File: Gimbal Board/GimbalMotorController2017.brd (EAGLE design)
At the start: 83.4 x 72.1 mm, 125 parts, among them J1 SL03THROUGH_HOLE, J3 APP_2POS_CONFIG5V_HORIZ, Q7 MOSFET-PCHANNEL, Q8 MOSFET-PCHANNEL, Q9 MOSFET-NCHANNELAO3404A, U1 NUP4201MR6, U2 MAX3232D, U3 CSD18533Q5A, U4 CSD18533Q5A, U5 CSD18533Q5A, U6 CSD18533Q5A, U7 CSD18533Q5A, U8 CSD18533Q5A

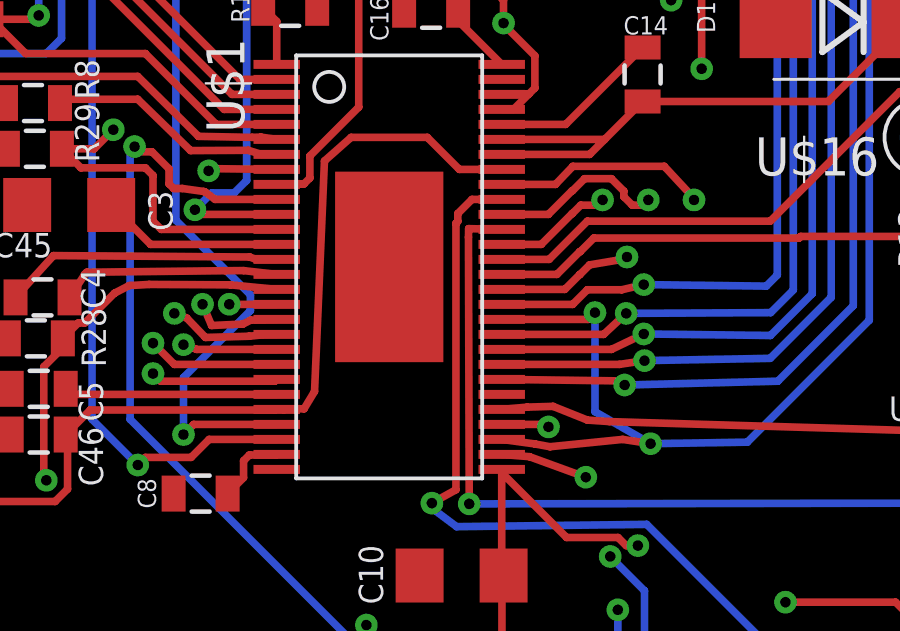
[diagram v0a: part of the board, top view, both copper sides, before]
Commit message: Board Updated for Board Review
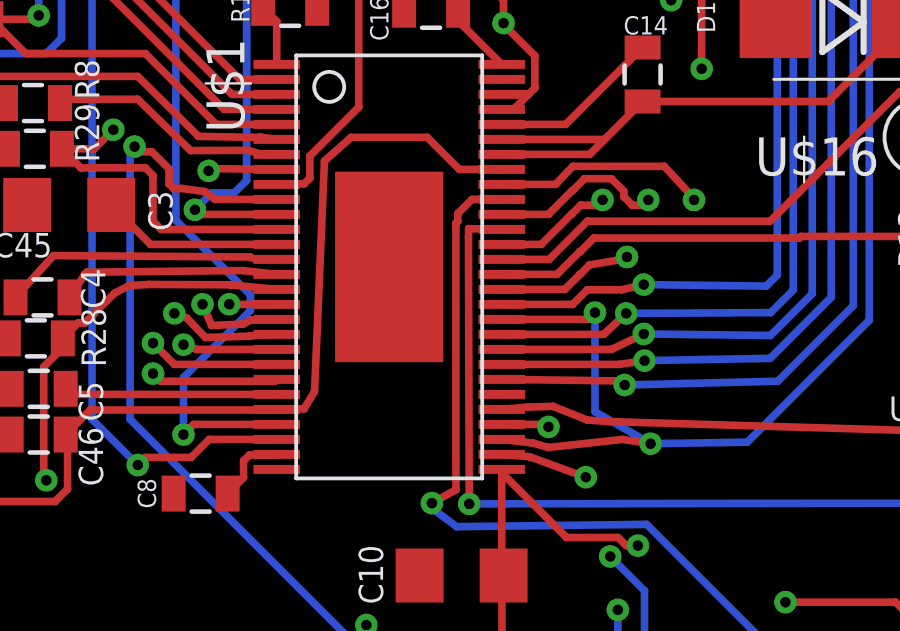
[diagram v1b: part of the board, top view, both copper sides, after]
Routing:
- net SDI: track 49.7 -> 48.9 mm
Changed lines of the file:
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@@
 <layers>
 <layer number="1" name="Top" color="4" fill="1" visible="yes" active="yes"/>
-<layer number="2" name="UpperMid" color="6" fill="1" visible="no" active="yes"/>
+<layer number="2" name="UpperMid" color="6" fill="1" visible="yes" active="yes"/>
 <layer number="3" name="Route3" color="4" fill="3" visible="no" active="no"/>
 <layer number="4" name="Route4" color="1" fill="4" visible="no" active="no"/>
@@
 <layer number="13" name="Route13" color="4" fill="5" visible="no" active="no"/>
 <layer number="14" name="Route14" color="1" fill="6" visible="no" active="no"/>
-<layer number="15" name="LowerMid" color="10" fill="1" visible="no" active="yes"/>
+<layer number="15" name="LowerMid" color="10" fill="1" visible="yes" active="yes"/>
 <layer number="16" name="Bottom" color="1" fill="1" visible="yes" active="yes"/>
 <layer number="17" name="Pads" color="2" fill="1" visible="yes" active="yes"/>
@@
 <wire x1="50.8" y1="3.81" x2="50.8" y2="4.80539375" width="0.254" layer="2"/>
 <wire x1="50.8" y1="4.80539375" x2="49.7078" y2="5.89759375" width="0.254" layer="2"/>
-<wire x1="49.7078" y1="5.89759375" x2="49.7078" y2="13.04436875" width="0.254" layer="2"/>
-<wire x1="49.7078" y1="13.04436875" x2="42.2176" y2="20.53456875" width="0.254" layer="2"/>
+<wire x1="49.7078" y1="5.89759375" x2="49.4538" y2="13.04436875" width="0.254" layer="2"/>
+<wire x1="49.4538" y1="13.04436875" x2="42.2176" y2="20.53456875" width="0.254" layer="2"/>
 <wire x1="42.2176" y1="27.8864" x2="42.164" y2="27.94" width="0.254" layer="2"/>
 <wire x1="42.2176" y1="20.53456875" x2="42.2176" y2="27.8864" width="0.254" layer="2"/>
@@
 <wire x1="47.32414375" y1="28.1698" x2="47.30434375" y2="28.15" width="0.254" layer="1"/>
 <wire x1="48.1552" y1="29.09754375" x2="48.1552" y2="28.363225" width="0.254" layer="1"/>
-<wire x1="47.961775" y1="28.1698" x2="47.0698" y2="28.1698" width="0.254" layer="1"/>
+<wire x1="47.32414375" y1="28.1698" x2="47.0698" y2="28.1698" width="0.254" layer="1"/>
 <wire x1="47.0698" y1="28.1698" x2="47.05" y2="28.15" width="0.254" layer="1"/>
 </signal>
@@
 <wire x1="73.8615" y1="45.43425" x2="73.8615" y2="47.01375" width="0.254" layer="1"/>
 <wire x1="73.50425" y1="47.371" x2="73.8615" y2="47.01375" width="0.254" layer="1"/>
-<wire x1="54.55" y1="19.65" x2="55.661" y2="19.4976" width="0.254" layer="1"/>
-<wire x1="55.661" y1="19.4976" x2="56.1594" y2="19.4056" width="0.254" layer="1"/>
-<wire x1="56.1594" y1="19.4056" x2="58.582" y2="19.65" width="0.254" layer="1"/>
+<wire x1="54.55" y1="19.65" x2="55.6102" y2="19.523" width="0.254" layer="1"/>
+<wire x1="55.6102" y1="19.523" x2="56.1086" y2="19.3802" width="0.254" layer="1"/>
+<wire x1="56.1086" y1="19.3802" x2="58.582" y2="19.65" width="0.254" layer="1"/>
 <wire x1="58.582" y1="19.65" x2="59.5122" y2="19.5072" width="0.254" layer="1"/>
 <via x="59.5122" y="19.5072" extent="1-16" drill="0.35"/>
